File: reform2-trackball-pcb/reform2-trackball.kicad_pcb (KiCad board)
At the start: 2 copper layers, 83.4 x 59 mm, 42 parts, among them J1 Conn_USB, J2 Conn_01x06_Female, SW1 Choc, SW2 Choc, SW3 Choc, SW4 Choc, SW5 Choc, SW6 SW_RST, SW7 SW_HWB, U1 ATmega32U2-AU, U2 TLV75533PDBV, Y1 Crystal_GND24

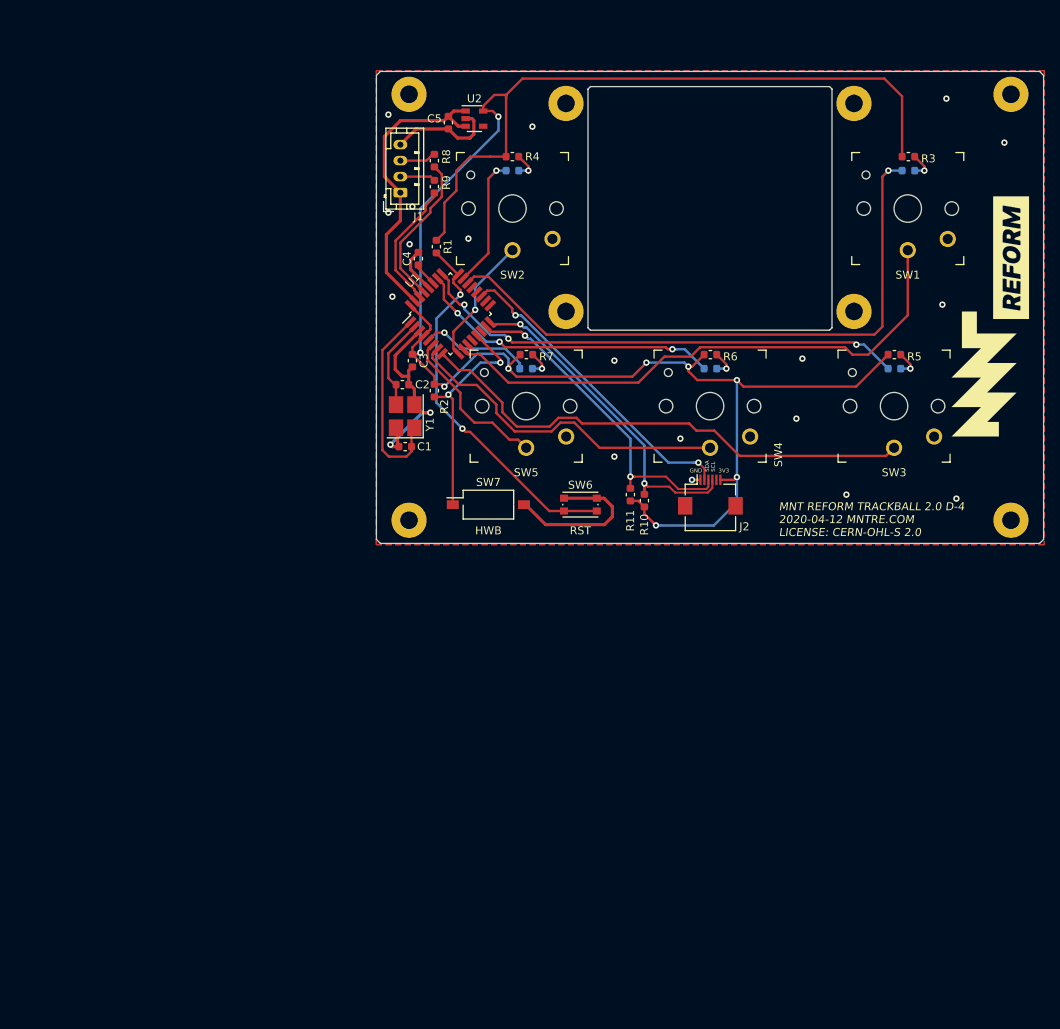
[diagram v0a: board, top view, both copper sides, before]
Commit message: new pcb
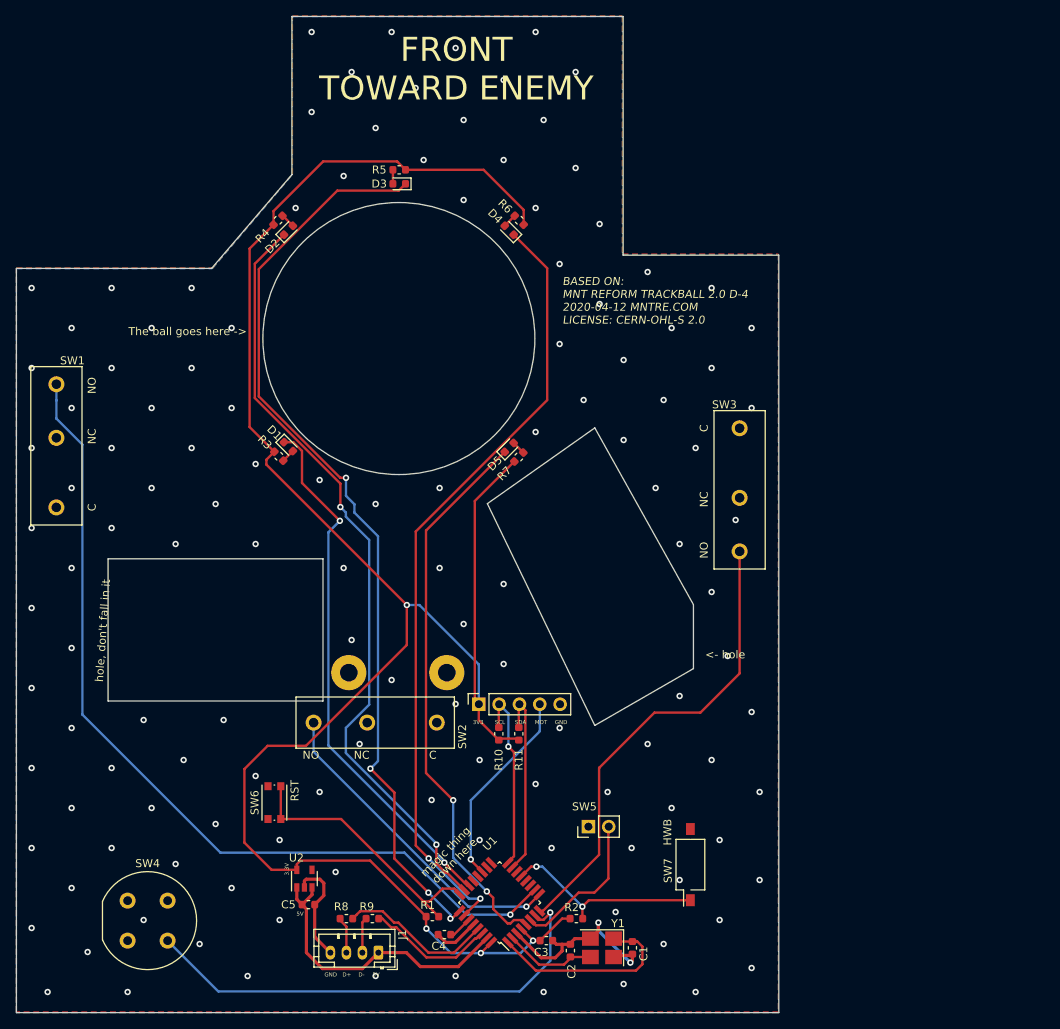
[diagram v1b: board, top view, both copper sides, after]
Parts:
- removed MK10, MK11, MK12, MK5, MK6, MK9: Mounting_Hole, MountingHole:MountingHole_2.2mm_M2_Pad
- removed MK13: LOGO, reform2-motherboard:mntreform
- D1, D2, D3, D4, D5: moved to F.Cu
- J2: value Conn_01x06_Female -> Conn_01x05_Female; footprint Connector_FFC-FPC:Hirose_FH12-6S-0.5SH_1x06-1MP_P0.50mm_Horizontal -> Connector_PinSocket_2.54mm:PinSocket_1x05_P2.54mm_Vertical
- SW1: value Choc -> left; footprint keyswitches:PG1350 -> d_switchs:SubminiatureSPDT; moved to F.Cu
- SW2: value Choc -> middle; footprint keyswitches:PG1350 -> d_switchs:SubminiatureSPDT; moved to F.Cu
- SW3: value Choc -> right; footprint keyswitches:PG1350 -> d_switchs:SubminiatureSPDT; moved to F.Cu
- SW4: value Choc -> btn4; footprint keyswitches:PG1350 -> Button_Switch_THT:Push_E-Switch_KS01Q01; moved to F.Cu
- SW5: value Choc -> btn5; footprint keyswitches:PG1350 -> Connector_PinHeader_2.54mm:PinHeader_1x02_P2.54mm_Vertical; moved to F.Cu
- moved SW1 112.8 mm to (69.0, 104.6), turned to 90 degrees
- moved C5 99.3 mm to (100.5, 154.2), turned to 0 degrees
- moved U2 97.3 mm to (100.0, 151.0), turned to 90 degrees
- moved R8 95.4 mm to (105.2, 156.0), turned to 0 degrees
- moved J1 95.0 mm to (109.2, 160.2), turned to 180 degrees
- moved R9 91.8 mm to (108.5, 156.0), turned to 180 degrees
- moved SW4 91.8 mm to (82.9, 153.8), turned to 270 degrees
- moved R3 87.2 mm to (96.8, 98.2), turned to 135 degrees
- moved MK7 84.9 mm to (105.5, 125.2)
- moved D1 84.8 mm to (98.0, 97.0), turned to 315 degrees
- moved C4 84.6 mm to (117.5, 158.0), turned to 180 degrees
- moved R1 83.8 mm to (116.0, 155.8), turned to 0 degrees
- moved C3 74.4 mm to (130.2, 158.8), turned to 0 degrees
- moved U1 73.9 mm to (124.4, 154.0), turned to 135 degrees
- moved C2 73.8 mm to (133.2, 160.0), turned to 270 degrees
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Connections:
- J2 pad 1: GND -> +3V3
- J2 pad 2: MT -> SCL
- J2 pad 4: SCL -> MT
- J2 pad 5: Net-(J2-Pad5) -> GND
- SW1 pad 1: Net-(SW1-Pad1) -> GND
- SW1 pad 2: GND -> Net-(SW1-Pad2)
- SW2 pad 1: Net-(SW2-Pad1) -> GND
- SW2 pad 2: GND -> Net-(SW2-Pad2)
- SW3 pad 1: Net-(SW3-Pad1) -> GND
- SW3 pad 2: GND -> Net-(SW3-Pad2)
- SW4 pad 1: Net-(SW4-Pad1) -> GND
- SW4 pad 2: GND -> Net-(SW4-Pad2)
- SW5 pad 1: Net-(SW5-Pad1) -> GND
- SW5 pad 2: GND -> Net-(SW5-Pad2)
- U1 pad 10: Net-(SW1-Pad1) -> Net-(SW1-Pad3)
- U1 pad 6: Net-(SW5-Pad1) -> Net-(SW5-Pad2)
- U1 pad 7: Net-(SW4-Pad1) -> Net-(SW4-Pad2)
- U1 pad 8: Net-(SW3-Pad1) -> Net-(SW3-Pad3)
- U1 pad 9: Net-(SW2-Pad1) -> Net-(SW2-Pad3)
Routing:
- net Net-(SW1-Pad3): track 0.00 -> 110.9 mm, vias 0 -> 1
- net Net-(D2-Pad1): track 16.4 -> 96.8 mm, vias 1 -> 2
- net Net-(SW1-Pad1): track 69.7 -> 0.00 mm
- net Net-(SW3-Pad1): track 63.8 -> 0.00 mm
- net Net-(SW4-Pad2): track 0.00 -> 60.6 mm, vias 0 -> 1
- net Net-(D4-Pad1): track 39.1 -> 98.7 mm, vias 3 -> 2
- net Net-(SW3-Pad3): track 0.00 -> 58.9 mm
- net Net-(D5-Pad1): track 14.3 -> 70.0 mm, vias 1 -> 2
- net Net-(D3-Pad1): track 61.9 -> 116.6 mm, vias 3 -> 4
- net Net-(SW4-Pad1): track 42.3 -> 0.00 mm
- net Net-(SW2-Pad3): track 0.00 -> 40.5 mm, vias 0 -> 1
- net GND: track 66.4 -> 45.1 mm, vias 20 -> 133
- net Net-(SW5-Pad1): track 20.2 -> 0.00 mm
- net SCL: track 43.0 -> 23.8 mm, vias 2 -> 1
- net Net-(SW5-Pad2): track 0.00 -> 19.0 mm
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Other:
- board size 83.4 x 59 mm -> 95.3 x 124.5 mm
- board text added: "1.6mm pcb"
- board text added: "10mm"
- board text added: "1mm sensor"
- board text added: "3.3V"
- board text added: "4mm margin 1mm minimum"
- board text added: "5V"
- board text added: "<- hole"
- board text added: "BASED ON: MNT REFORM TRACKBALL 2.0 D-4 2020-04-12 MNTRE.COM LICENSE: CERN-OHL-S 2.0"
- board text added: "D+"
- board text added: "D-"
- board text added: "FRONT TOWARD ENEMY"
- board text added: "MOT"
- board text added: "The ball goes here ->"
- board text added: "hole, don't fall in it"
- board text added: "magic thing down here"
- board text added: "size of ball"
- board text added: "total board width"
- board text added: "width btw holes"
- board text removed: "MNT REFORM TRACKBALL 2.0 D-4 2020-04-12 MNTRE.COM LICENSE: CERN-OHL-S 2.0"
